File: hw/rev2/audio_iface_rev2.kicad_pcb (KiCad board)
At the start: 4 copper layers, 57.4 x 42.8 mm, 79 parts, among them J1 USB_B_Micro, J2 Conn_01x08, J3 Amphenol 20021122, J4 Screw_Terminal_01x02, U1 USBLC6-2SC6, U2 STM32H743VITx, U3 USB3300-EZK, U4 ADAU1772, U5 LP5907MFX-3.3, U6 LP5907MFX-1.8, U7 LP5907MFX-3.3, X1 DSC6011JE1A-024.0000, X2 DSC6011CI2A-012.2880

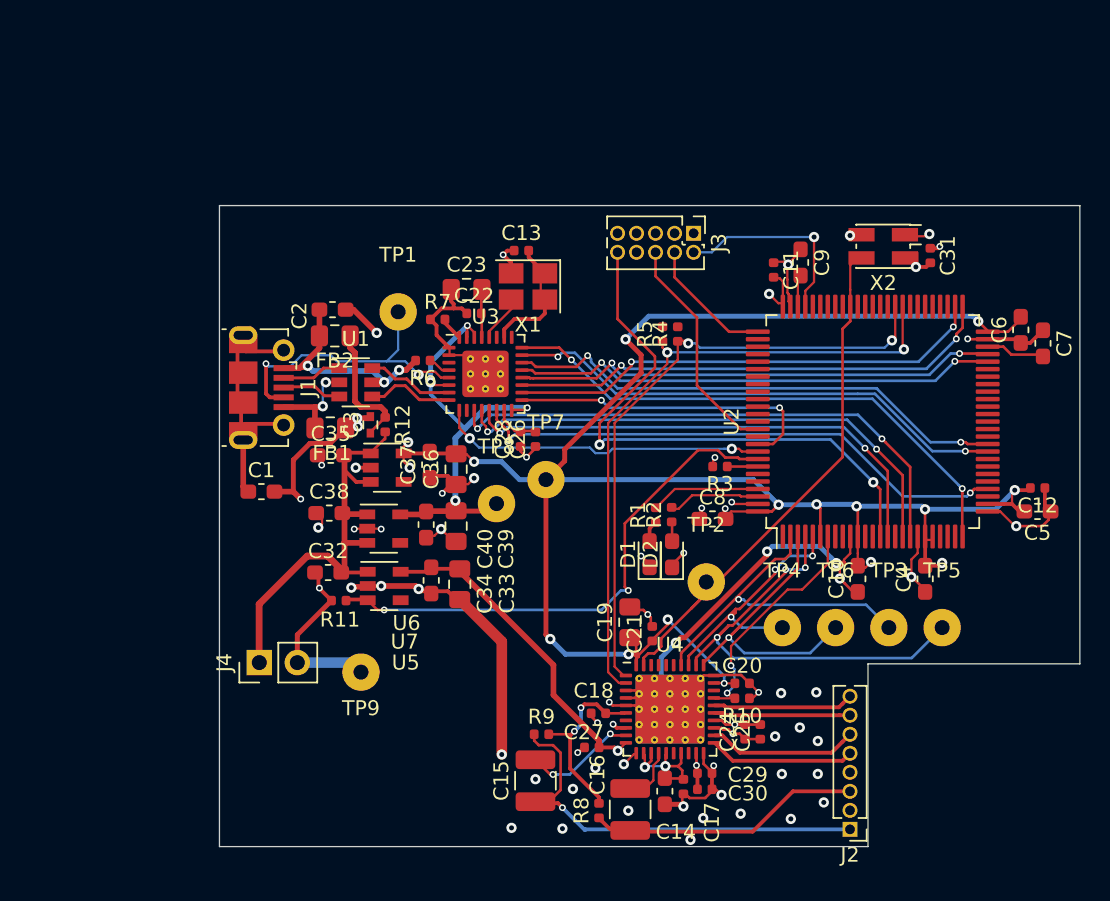
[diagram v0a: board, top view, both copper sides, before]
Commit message: Design nearly complete. One more check.
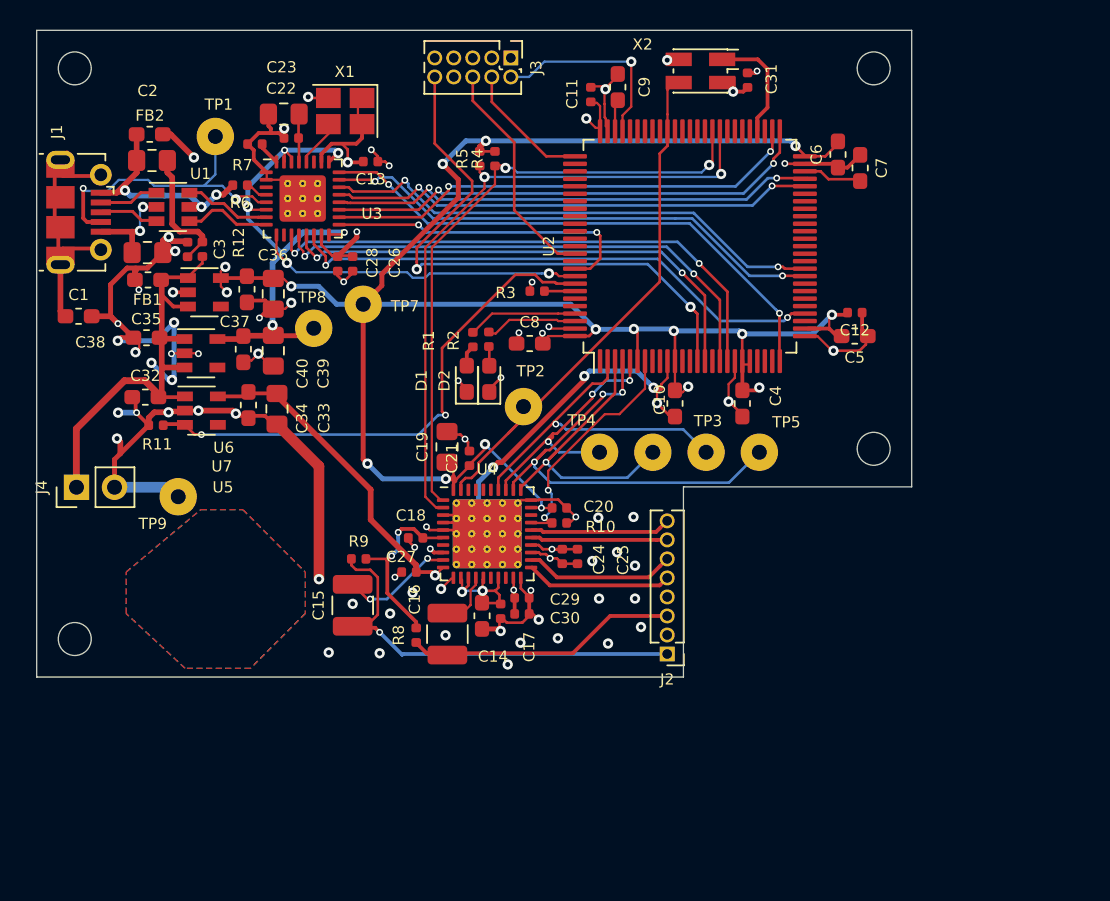
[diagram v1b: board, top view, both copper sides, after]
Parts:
- removed the G*** at (100.6, 99.3)
- added G***: LOGO, ear:LOGO, B.Cu at (88.4, 88.1)
- added G***: LOGO, ear:LOGO, F.Cu at (88.2, 88.3)
- added H1: MountingHole, MountingHole:MountingHole_2.2mm_M2, F.Cu at (78.7, 53.3)
- added H2: MountingHole, MountingHole:MountingHole_2.2mm_M2, F.Cu at (78.7, 91.4)
- added H3: MountingHole, MountingHole:MountingHole_2.2mm_M2, F.Cu at (132.1, 53.3)
- added H4: MountingHole, MountingHole:MountingHole_2.2mm_M2, F.Cu at (132.1, 78.7)
- C3: footprint Capacitors_SMD:C_0402 -> Capacitor_SMD:C_0402_1005Metric
- moved C11 16.9 mm to (113.2, 55.1)
- moved C12 16.9 mm to (130.8, 69.6)
- moved C15 16.9 mm to (97.3, 89.2)
- moved C18 16.9 mm to (101.5, 84.7)
- moved C2 16.9 mm to (83.7, 57.7)
- moved C20 16.9 mm to (111.1, 82.7)
- moved C21 16.9 mm to (105.1, 79.4)
- moved C22 16.9 mm to (93.2, 58.0)
- moved C23 16.9 mm to (92.7, 56.4)
- moved C24 16.9 mm to (111.3, 85.9)
- moved C25 16.9 mm to (112.3, 85.9)
- moved C27 16.9 mm to (101.1, 87.0)
- moved C29 16.9 mm to (108.6, 88.7)
- moved C30 16.9 mm to (108.6, 89.8)
- moved C31 16.9 mm to (123.7, 54.1)
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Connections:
- C1 pad 2: GNDD -> AGND
- C10 pad 1: GNDD -> AGND
- C11 pad 1: GNDD -> AGND
- C12 pad 1: GNDD -> AGND
- C13 pad 1: GNDD -> AGND
- C18 pad 2: GNDD -> AGND
- C19 pad 2: GNDD -> AGND
- C2 pad 2: GNDD -> AGND
- C20 pad 2: GNDD -> AGND
- C21 pad 2: GNDD -> AGND
- C22 pad 1: GNDD -> AGND
- C23 pad 1: GNDD -> AGND
- C26 pad 1: GNDD -> AGND
- C28 pad 1: GNDD -> AGND
- C3 pad 2: GNDD -> AGND
- C31 pad 1: GNDD -> AGND
- C32 pad 1: GND -> AGND
- C35 pad 1: GND -> AGND
- C36 pad 1: GND -> AGND
- C37 pad 1: GND -> AGND
- C38 pad 1: GND -> AGND
- C39 pad 1: GND -> AGND
- C4 pad 1: GNDD -> AGND
- C40 pad 1: GND -> AGND
- C5 pad 1: GNDD -> AGND
- C6 pad 1: GNDD -> AGND
- C7 pad 1: GNDD -> AGND
- C8 pad 1: GNDD -> AGND
- C9 pad 1: GNDD -> AGND
- D1 pad 1: GNDD -> AGND
- D2 pad 1: GNDD -> AGND
- FB1 pad 2: GNDD -> AGND
- J3 pad 3: GNDD -> AGND
- J3 pad 5: GNDD -> AGND
- J3 pad 7: (no net) -> Net-(J3-Pad7)
- J3 pad 8: (no net) -> Net-(J3-Pad8)
- J3 pad 9: GNDD -> AGND
- J4 pad 2: GND -> AGND
- R10 pad 1: GNDD -> AGND
- R11 pad 1: GND -> AGND
- R3 pad 2: GNDD -> AGND
- R4 pad 2: +3V -> +1V8
- R5 pad 2: +3V -> +1V8
- R7 pad 1: GNDD -> AGND
- TP9 pad 1: GND -> AGND
- U2 pad 1: (no net) -> Net-(U2-Pad1)
- U2 pad 10: GNDD -> AGND
- U2 pad 12: (no net) -> Net-(U2-Pad12)
- U2 pad 13: (no net) -> Net-(U2-Pad13)
- U2 pad 16: (no net) -> Net-(U2-Pad16)
- U2 pad 19: GNDD -> AGND
- U2 pad 22: (no net) -> Net-(U2-Pad22)
- U2 pad 23: (no net) -> Net-(U2-Pad23)
- U2 pad 24: (no net) -> Net-(U2-Pad24)
- U2 pad 26: GNDD -> AGND
- U2 pad 28: (no net) -> Net-(U2-Pad28)
- U2 pad 30: (no net) -> Net-(U2-Pad30)
- U2 pad 31: (no net) -> Net-(U2-Pad31)
- U2 pad 32: (no net) -> Net-(U2-Pad32)
- U2 pad 33: (no net) -> Net-(U2-Pad33)
- U2 pad 36: (no net) -> Net-(U2-Pad36)
- U2 pad 37: (no net) -> Net-(U2-Pad37)
- U2 pad 38: (no net) -> Net-(U2-Pad38)
- U2 pad 39: (no net) -> Net-(U2-Pad39)
- U2 pad 40: (no net) -> Net-(U2-Pad40)
- U2 pad 41: (no net) -> Net-(U2-Pad41)
- U2 pad 42: (no net) -> Net-(U2-Pad42)
- U2 pad 43: (no net) -> Net-(U2-Pad43)
- U2 pad 44: (no net) -> Net-(U2-Pad44)
- U2 pad 45: (no net) -> Net-(U2-Pad45)
- U2 pad 49: GNDD -> AGND
- U2 pad 53: (no net) -> Net-(U2-Pad53)
- U2 pad 54: (no net) -> /Microcontroller/MCLK_EN
- U2 pad 55: (no net) -> Net-(U2-Pad55)
- U2 pad 56: (no net) -> Net-(U2-Pad56)
- U2 pad 57: (no net) -> Net-(U2-Pad57)
- U2 pad 58: (no net) -> Net-(U2-Pad58)
- U2 pad 61: (no net) -> Net-(U2-Pad61)
- U2 pad 62: (no net) -> Net-(U2-Pad62)
- U2 pad 63: (no net) -> Net-(U2-Pad63)
- U2 pad 64: (no net) -> Net-(U2-Pad64)
- U2 pad 65: (no net) -> Net-(U2-Pad65)
- U2 pad 67: (no net) -> Net-(U2-Pad67)
- U2 pad 68: (no net) -> Net-(U2-Pad68)
- U2 pad 69: (no net) -> Net-(U2-Pad69)
- U2 pad 70: (no net) -> Net-(U2-Pad70)
- U2 pad 71: (no net) -> Net-(U2-Pad71)
- U2 pad 74: GNDD -> AGND
- U2 pad 77: (no net) -> Net-(U2-Pad77)
- U2 pad 78: (no net) -> Net-(U2-Pad78)
- U2 pad 79: (no net) -> Net-(U2-Pad79)
- U2 pad 8: (no net) -> Net-(U2-Pad8)
- U2 pad 80: (no net) -> Net-(U2-Pad80)
- U2 pad 81: (no net) -> Net-(U2-Pad81)
- U2 pad 82: (no net) -> Net-(U2-Pad82)
- U2 pad 83: (no net) -> Net-(U2-Pad83)
- U2 pad 84: (no net) -> Net-(U2-Pad84)
- U2 pad 85: (no net) -> Net-(U2-Pad85)
- U2 pad 86: (no net) -> Net-(U2-Pad86)
- U2 pad 87: (no net) -> Net-(U2-Pad87)
- U2 pad 88: (no net) -> Net-(U2-Pad88)
- U2 pad 9: (no net) -> Net-(U2-Pad9)
- U2 pad 90: (no net) -> Net-(U2-Pad90)
- U2 pad 95: (no net) -> Net-(U2-Pad95)
- U2 pad 96: (no net) -> Net-(U2-Pad96)
- U2 pad 99: GNDD -> AGND
- U3 pad 1: GNDD -> AGND
- U3 pad 10: (no net) -> Net-(U3-Pad10)
- U3 pad 2: GNDD -> AGND
- U3 pad 27: (no net) -> Net-(U3-Pad27)
- U3 pad 3: (no net) -> Net-(U3-Pad3)
- U3 pad 33: GNDD -> AGND
- U4 pad 16: (no net) -> Net-(U4-Pad16)
- U4 pad 18: (no net) -> Net-(U4-Pad18)
- U4 pad 28: (no net) -> Net-(U4-Pad28)
- U4 pad 3: GNDD -> AGND
- U4 pad 30: GNDD -> AGND
- U4 pad 35: (no net) -> Net-(U4-Pad35)
- U4 pad 36: (no net) -> Net-(U4-Pad36)
- U4 pad 37: (no net) -> Net-(U4-Pad37)
- U4 pad 38: (no net) -> Net-(U4-Pad38)
- U4 pad 4: GNDD -> AGND
- U4 pad 41: GNDD -> AGND
- U4 pad 5: GNDD -> AGND
- U4 pad 7: (no net) -> Net-(U4-Pad7)
- U5 pad 4: (no net) -> Net-(U5-Pad4)
- U6 pad 2: GND -> AGND
- U6 pad 4: (no net) -> Net-(U6-Pad4)
- U7 pad 2: GND -> AGND
- U7 pad 4: (no net) -> Net-(U7-Pad4)
- X1 pad 2: GNDD -> AGND
- X2 pad 1: (no net) -> /Microcontroller/MCLK_EN
- X2 pad 2: GNDD -> AGND
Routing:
- net AGND: track 33.5 -> 166.6 mm, vias 28 -> 71
- net GNDD: track 89.8 -> 0.00 mm, vias 25 -> 0
- net GND: track 23.4 -> 0.00 mm, vias 9 -> 0
- net /Microcontroller/1V8_USB: track 10.9 -> 19.1 mm, vias 0 -> 2
- net /Microcontroller/MCLK_EN: track 0.00 -> 7.73 mm
- net +3V3: track 30.3 -> 34.9 mm, vias 4 -> 5
- net +1V8: track 144.1 -> 146.0 mm, vias 19 -> 20
- net (no net): track 0.86 -> 0.00 mm, vias 1 -> 0
- added copper zone on B.Cu, net (none)
- added copper zone on F.Cu, net (none)
- removed copper zone on Inner2.Cu, net GND
- removed copper zone on Inner2.Cu, net GNDD
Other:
- board size 57.4 x 42.8 mm -> 58.4 x 43.2 mm
